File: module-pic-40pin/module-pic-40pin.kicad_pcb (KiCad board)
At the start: 2 copper layers, 104.7 x 73.3 mm, 23 parts, among them J1 rb0_enable, J2 power_input, J3 power, J4 icsp, J5 ANALOG, J6 PORTC, J7 PORTB, J8 PORTD, SW1 EXT_INT0, SW2 RESET, U1 PIC16F877A-IP, Y1 20MHz

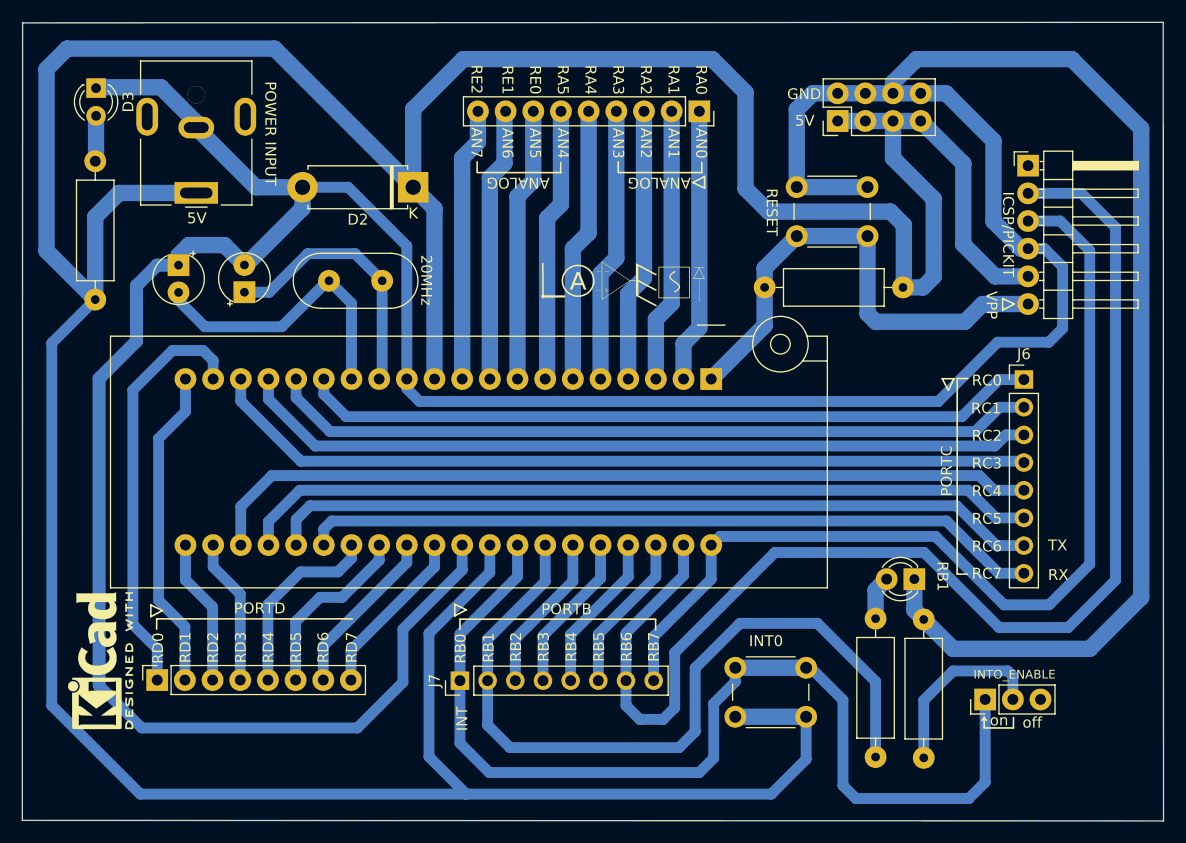
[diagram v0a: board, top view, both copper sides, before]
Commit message: update module-pic-40pin project
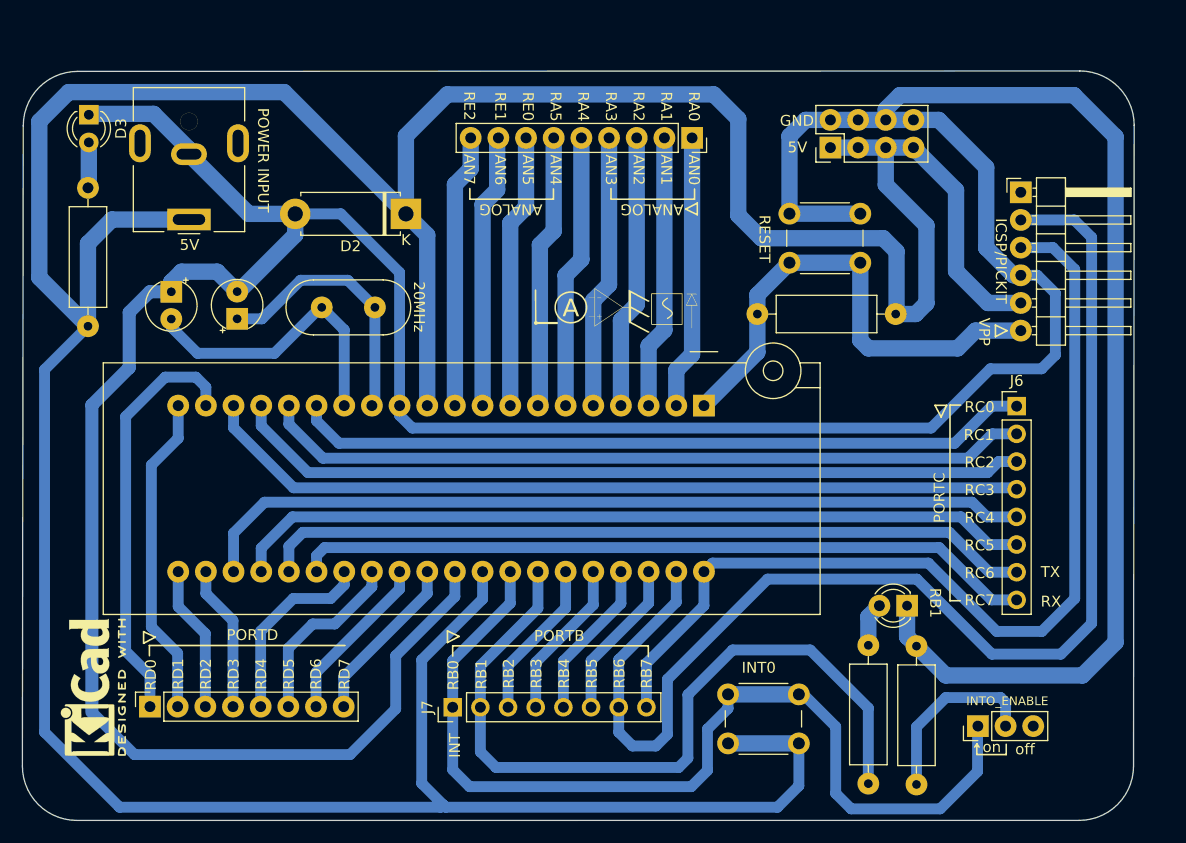
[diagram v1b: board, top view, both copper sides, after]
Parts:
- moved J1 2.53 mm to (143.3, 90.4)
- moved R1 2.53 mm to (137.7, 95.8)
- moved G*** 2.53 mm to (110.1, 52.3)
- moved J5 2.53 mm to (117.1, 36.4)
- moved REF** 2.53 mm to (62.1, 86.8)
- moved C1 2.53 mm to (75.3, 53.0)
- moved D1 2.53 mm to (136.8, 79.4)
- moved J3 2.53 mm to (129.8, 37.3)
- moved J4 2.53 mm to (147.3, 41.4)
- moved J6 2.53 mm to (146.9, 61.0)
- moved J8 2.53 mm to (67.3, 88.6)
- moved SW2 2.53 mm to (126.0, 43.4)
- moved U1 2.53 mm to (118.2, 61.0)
- moved D3 2.53 mm to (61.7, 34.3)
- moved J2 2.53 mm to (70.9, 43.9)
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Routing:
- net +5V: track 366.9 -> 360.7 mm
- net /RB0: track 95.2 -> 89.2 mm
- net GND: track 370.7 -> 368.6 mm
- net /RB6: track 117.9 -> 116.7 mm
- net /RB7: track 89.4 -> 88.8 mm
- net /RB1: track 72.5 -> 72.0 mm
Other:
- board size 104.7 x 73.3 mm -> 102.1 x 68.8 mm

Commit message: update module-pic-40pin
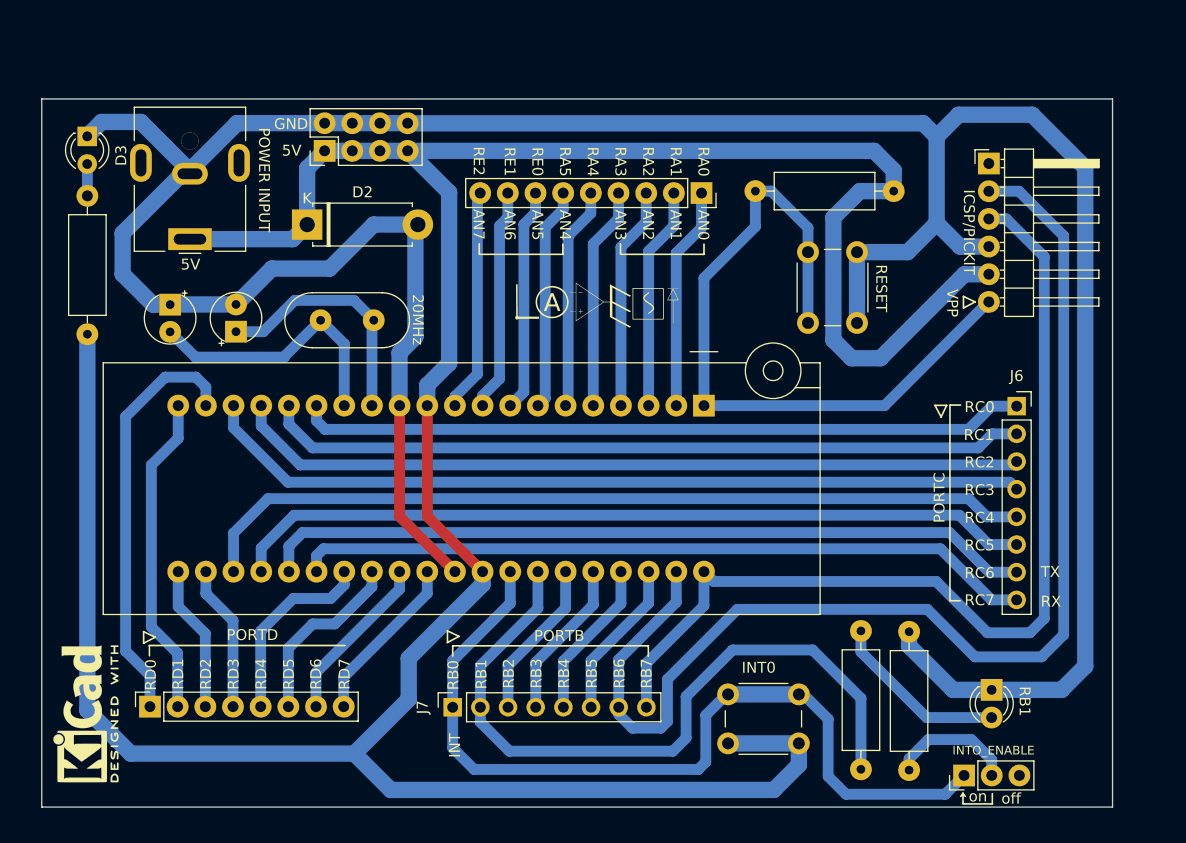
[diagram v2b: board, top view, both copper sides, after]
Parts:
- J6, J7: footprint Connector_PinHeader_2.54mm:PinHeader_1x08_P2.54mm_Vertical -> Connector_PinSocket_2.54mm:PinSocket_1x08_P2.54mm_Vertical
- moved J3 46.4 mm to (83.4, 37.6)
- moved R4 11.3 mm to (122.9, 41.3)
- moved D1 11.0 mm to (144.6, 87.1), turned to -90 degrees
- moved D2 9.12 mm to (81.8, 44.4), turned to 0 degrees
- moved SW2 7.13 mm to (132.2, 46.9), turned to -90 degrees
- moved J5 5.14 mm to (118.0, 41.5)
- moved J1 4.71 mm to (142.1, 94.9)
- moved J4 3.94 mm to (144.3, 38.8)
- moved REF** 2.53 mm to (61.4, 89.3)
- moved D3 1.99 mm to (61.6, 36.3)
- moved J2 1.80 mm to (71.0, 45.7)
- moved G*** 1.79 mm to (108.4, 51.8)
- moved R2 1.48 mm to (132.6, 81.7)
- moved R1 1.48 mm to (137.0, 94.4)
- moved C1 1.19 mm to (75.2, 54.2)
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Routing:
- net GND: track 368.6 -> 272.6 mm
- net +5V: track 360.7 -> 287.0 mm
- net /VPP: track 45.7 -> 67.2 mm
- net Net-(D1-Pad2): track 4.05 -> 16.4 mm
- net /RB0: track 89.2 -> 79.1 mm
- net /RB1: track 72.0 -> 66.5 mm
- net /RB6: track 116.7 -> 111.3 mm
- net Net-(J1-Pad2): track 16.9 -> 11.6 mm
- net /RA5: track 25.2 -> 20.5 mm
- net /RE2: track 25.2 -> 20.5 mm
- net /RA2: track 25.2 -> 20.5 mm
- net /RA0: track 25.2 -> 20.5 mm
- net /RA1: track 25.2 -> 20.5 mm
- net /RA3: track 25.2 -> 20.5 mm
- net /RE1: track 25.2 -> 20.7 mm
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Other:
- board size 102.1 x 68.8 mm -> 98.3 x 65 mm
- board text removed: "ANALOG"
